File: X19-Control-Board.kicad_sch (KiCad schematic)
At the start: 28 parts, among them U1 STM32C542CCT6, U2 TCAN1044VDRQ1, Y2 ECS-400-18-33-JGN-TR

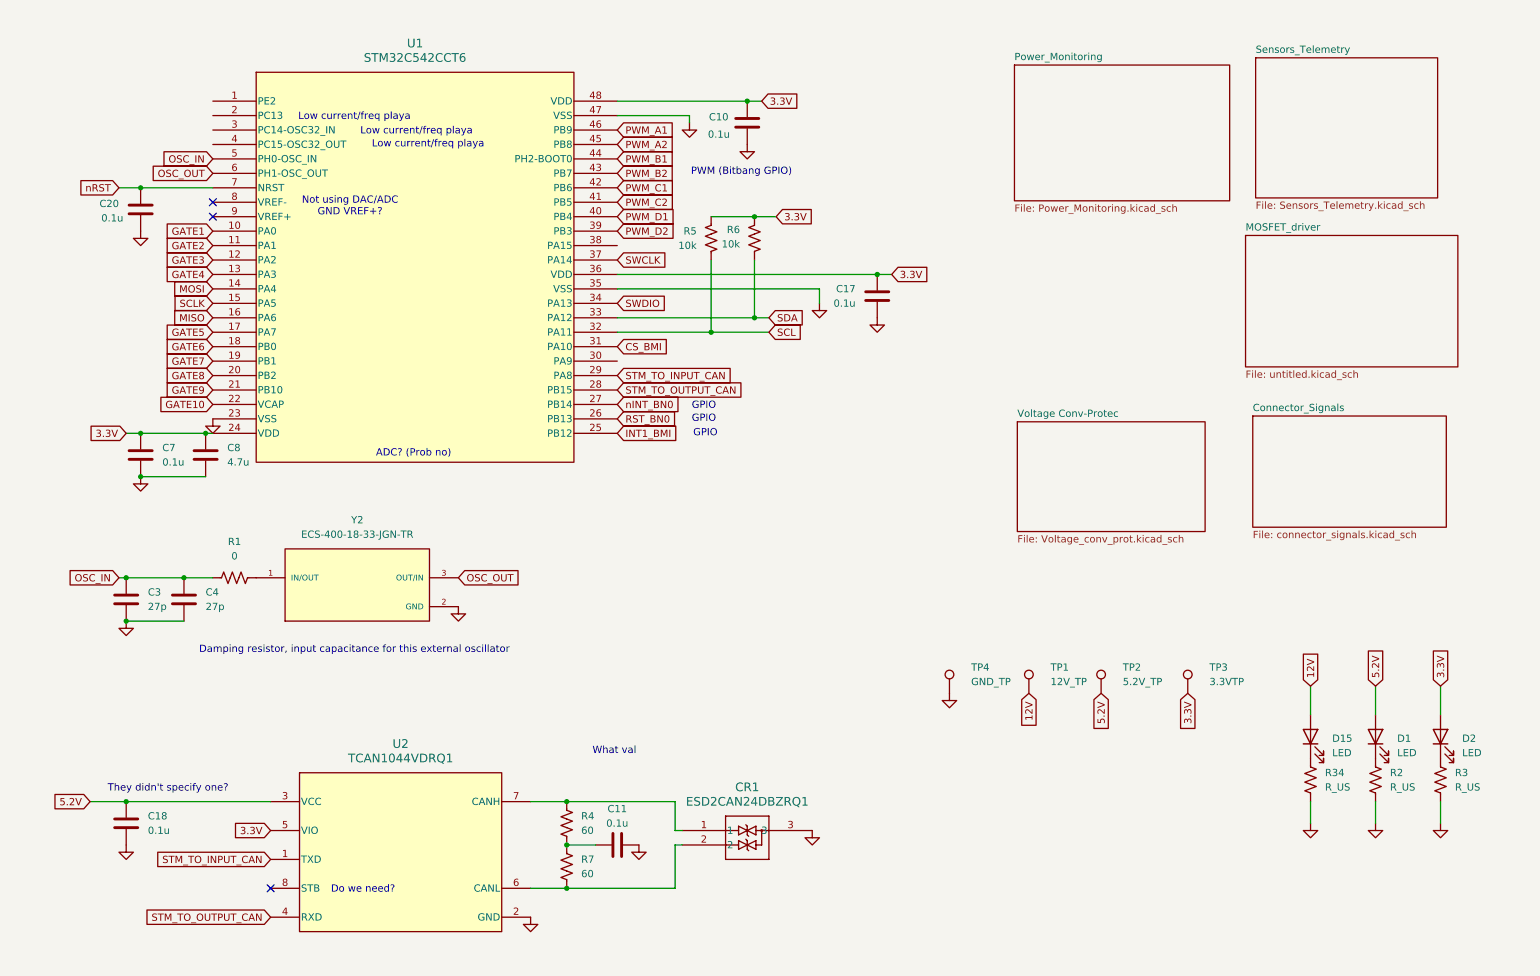
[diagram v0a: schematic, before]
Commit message: Final v1
Finished making it look nice, looking for feedback
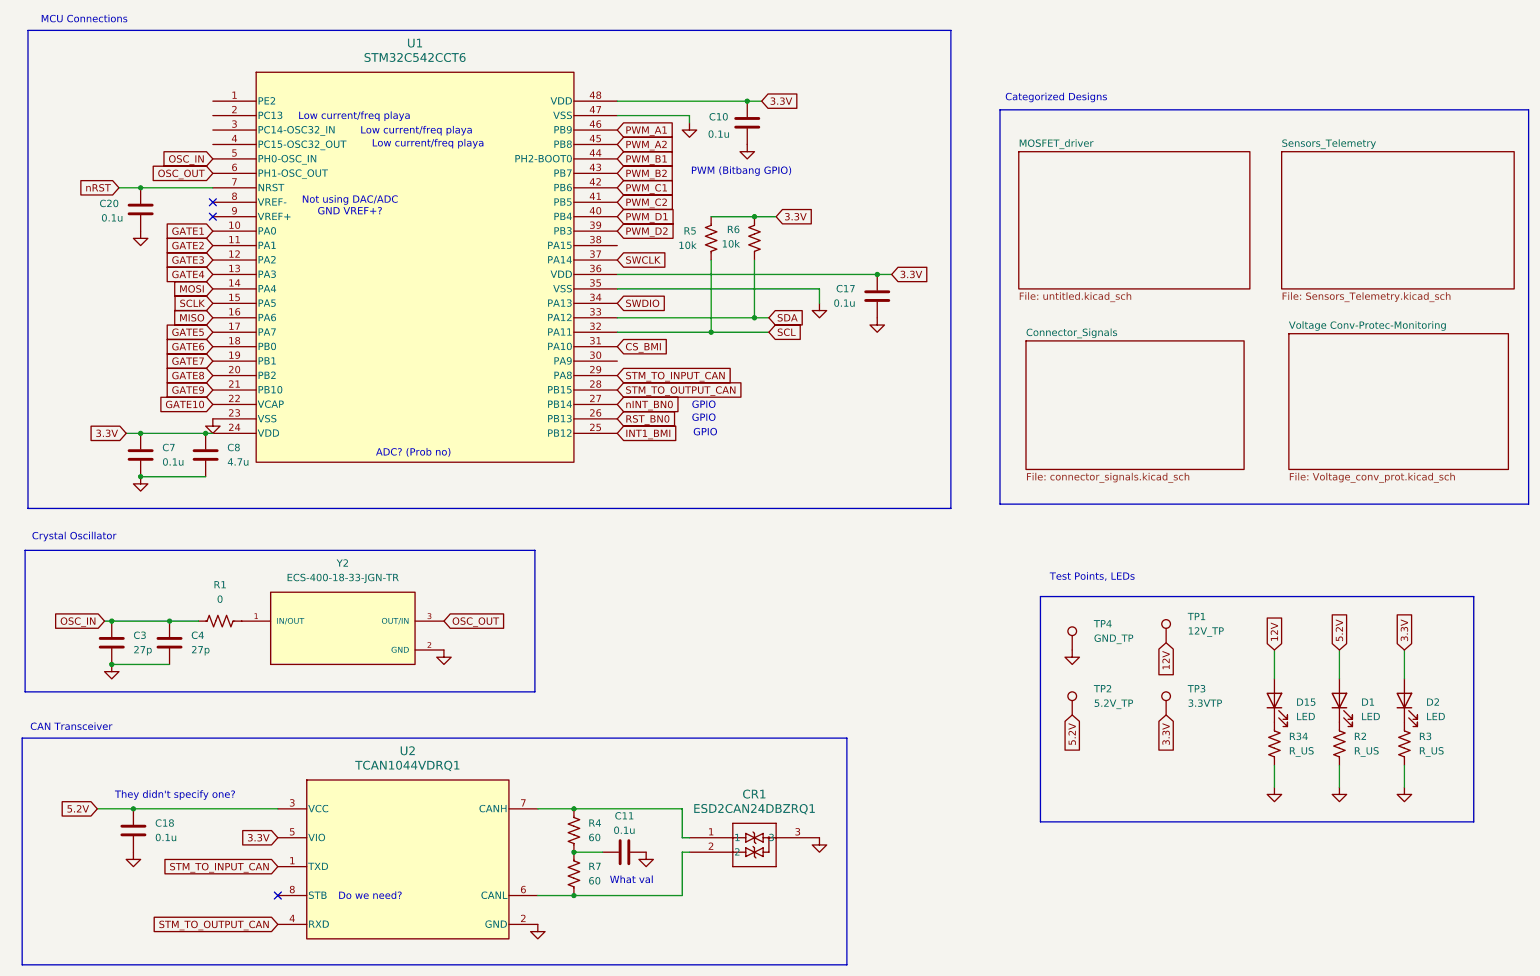
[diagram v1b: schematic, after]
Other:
- sheet Voltage Conv-Protec renamed Voltage Conv-Protec-Monitoring
- removed sheet Power_Monitoring
- note added: "CAN Transceiver"
- note added: "Categorized Designs"
- note added: "Crystal Oscillator"
- note added: "MCU Connections"
- note added: "Test Points, LEDs"
- note removed: "Damping resistor, input capacitance for this external oscillator"
- moved on the sheet: C11, C18, C3, C4, CR1, D1, D15, D2, R1, R2, R3, R34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
